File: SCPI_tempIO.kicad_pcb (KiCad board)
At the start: 2 copper layers, 40.3 x 21.4 mm, 30 parts, among them J1 Conn_ARM_JTAG_SWD_10, J2 Conn_02x05_Counter_Clockwise, J3 USB_C_Receptacle_USB2.0_14P, J4 Conn_01x04_Pin, J5 Conn_01x04_Pin, SW1 SW_SPST, U1 STM32G070KBTx, U2 AP2112K-3.3, U3 SHT4x

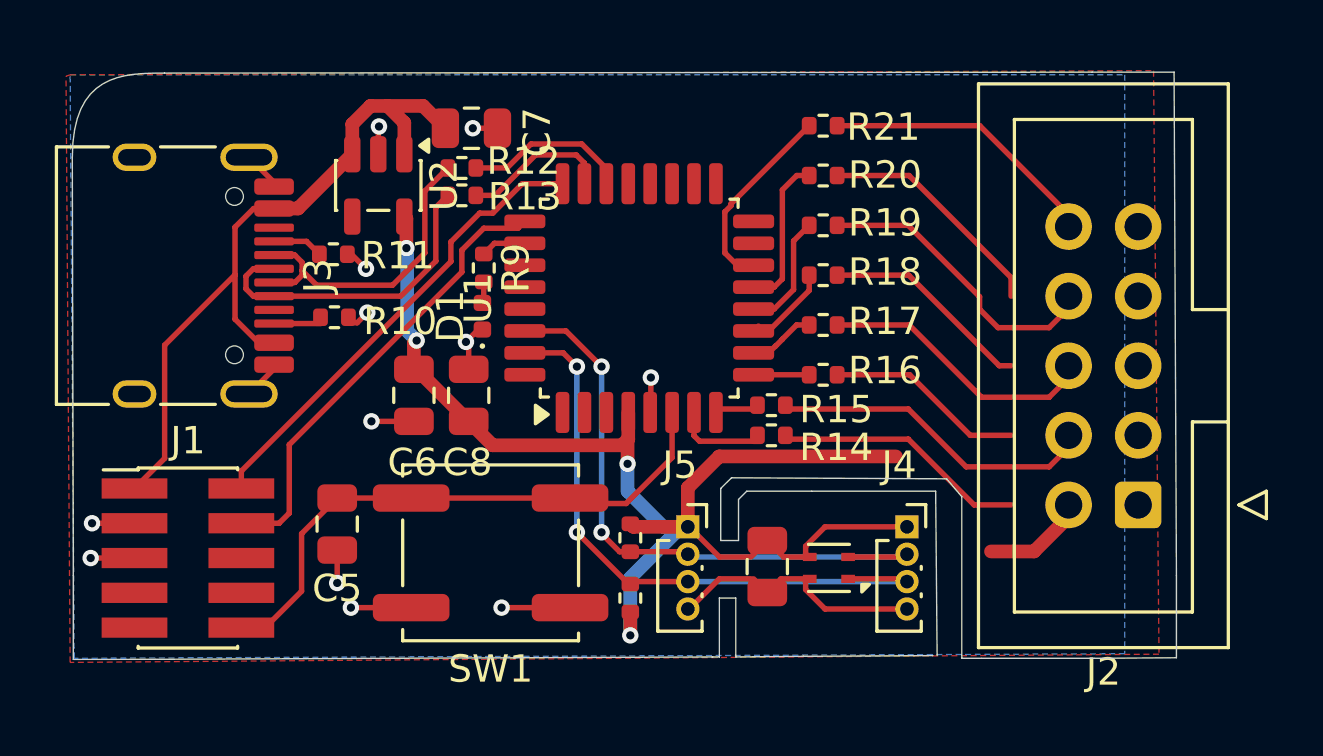
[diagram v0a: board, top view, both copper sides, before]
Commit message: sent to JLC noodleUSBp16
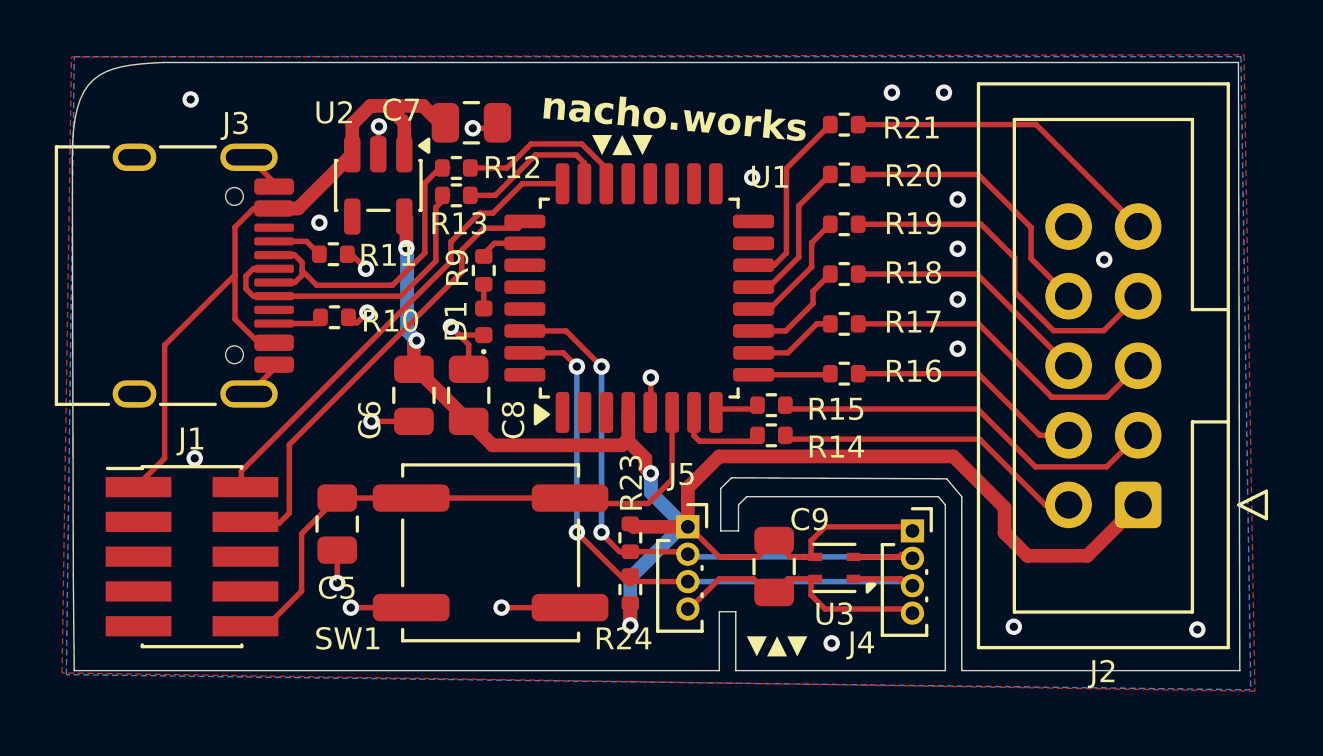
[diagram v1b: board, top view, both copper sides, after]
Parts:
- added G***: LOGO, LOGO, B.Cu at (89.9, 45.9)
- moved R16 0.77 mm to (90.0, 47.9)
- moved R17 0.77 mm to (90.0, 46.1)
- moved R18 0.77 mm to (90.0, 44.3)
- moved R19 0.77 mm to (90.0, 42.5)
- moved R20 0.77 mm to (90.0, 40.6)
- moved R21 0.77 mm to (90.0, 38.8)
- moved R24 0.31 mm to (82.2, 55.8)
- moved J4 0.25 mm to (92.5, 53.6)
- moved C9 0.25 mm to (87.5, 55.0)
- moved D1 0.21 mm to (76.8, 46.0)
- moved C7 0.20 mm to (76.4, 38.8)
- moved R12 0.20 mm to (75.8, 40.4)
- moved R13 0.20 mm to (75.8, 41.4)
- moved U3 0.20 mm to (89.7, 55.0)
- moved J1 0.16 mm to (66.2, 54.6)
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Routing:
- net /3v3: track 47.8 -> 58.4 mm
- net Net-(J2-Pin_3): track 12.2 -> 14.3 mm
- net Net-(J2-Pin_7): track 11.2 -> 13.1 mm
- net Net-(J2-Pin_2): track 13.3 -> 11.4 mm
- net Net-(J2-Pin_8): track 8.57 -> 10.3 mm
- net GND: track 30.4 -> 28.7 mm, vias 12 -> 24
- net Net-(J2-Pin_4): track 7.27 -> 8.61 mm
- net Net-(J2-Pin_6): track 7.72 -> 9.07 mm
- net Net-(J2-Pin_5): track 10.5 -> 11.8 mm
- net Net-(J2-Pin_9): track 10.4 -> 11.8 mm
- net Net-(U1-PA2): track 2.03 -> 2.82 mm
- net Net-(U1-PA3): track 2.55 -> 3.33 mm
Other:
- board size 40.3 x 21.4 mm -> 42.6 x 22.2 mm
- board text added: "SCPI-TEMPIO"
- board text added: "for all your temperature, humidity and other IO needs. Break off the SHT40 part and connect it using a 4 lead wire for more flexibility."
- board text added: "nacho.works"
- board text added: "▼▲▼"
